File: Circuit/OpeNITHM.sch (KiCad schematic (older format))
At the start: 59 parts, among them J1 Conn_01x12, J2 Conn_01x12, J3 Conn_01x08, J4 Conn_01x11, J5 Conn_01x08, J6 Conn_01x11, J7 Conn_01x04

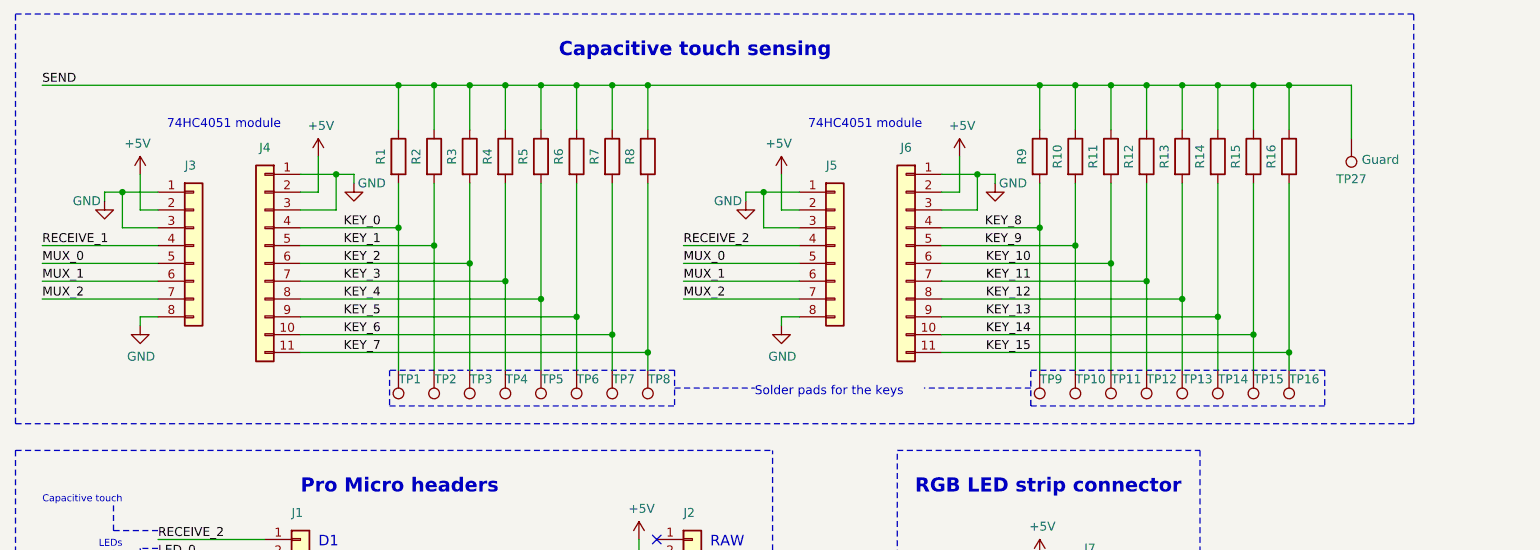
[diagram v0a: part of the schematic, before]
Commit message: Fix schematic files
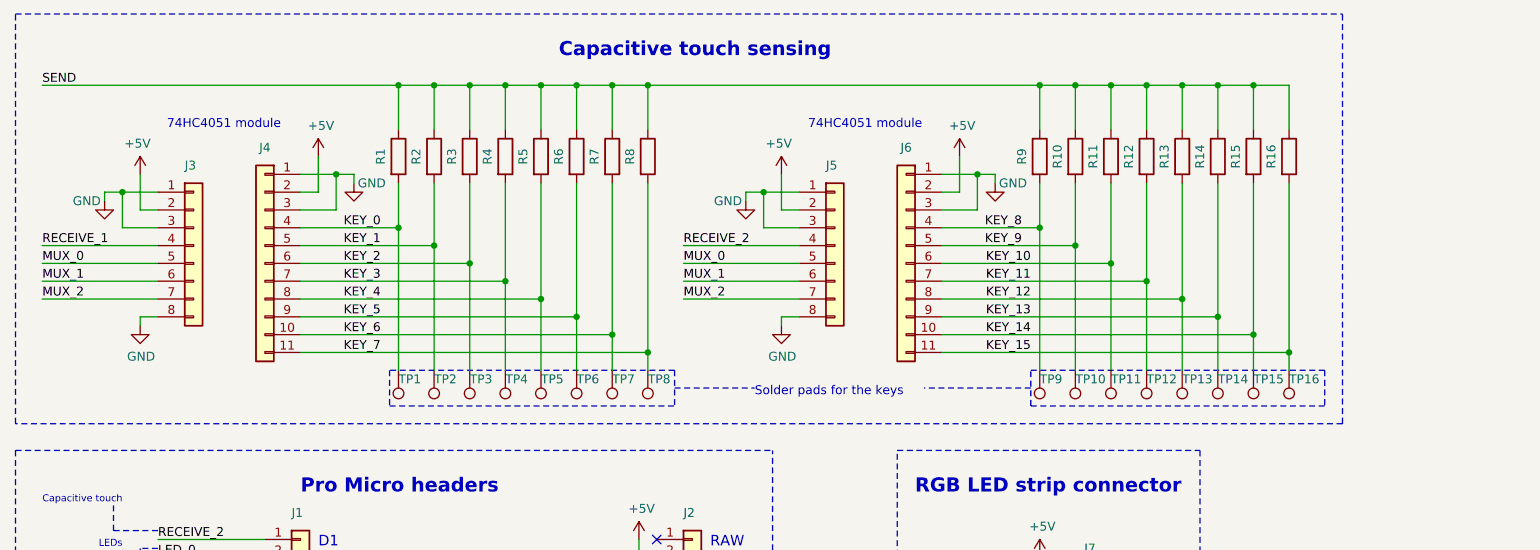
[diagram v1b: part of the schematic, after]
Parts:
- removed TP27: Guard, Connector_Wire:SolderWirePad_1x01_Drill1mm, symbol Connector:TestPoint
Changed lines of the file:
@@
 	9100 1200 9100 1450
+Wire Wire Line
+	9300 1200 9300 1450
 Wire Wire Line
 	9500 1200 9500 1450
@@
 Text Label 6100 2100 0    50   ~ 0
 RECEIVE_2
+Wire Wire Line
+	5900 1200 8100 1200
 Connection ~ 5900 1200
 Connection ~ 8100 1200
@@
 	3050 2550 3050 2500
 Wire Notes Line
-	10200 3100 10200 800
+	2350 800  9800 800
+Wire Notes Line
+	9800 3100 9800 800
+Wire Notes Line
+	9800 3100 2350 3100
 Wire Notes Line
 	2350 3100 2350 800
@@
 Wire Notes Line
 	2350 3250 6600 3250
-Wire Wire Line
-	5900 1200 8100 1200
-Wire Wire Line
-	9300 1200 9300 1450
-Connection ~ 9500 1200
-Wire Notes Line
-	2350 800  10200 800
-Wire Notes Line
-	2350 3100 10200 3100
-Wire Wire Line
-	9850 1200 9850 1500
-Wire Wire Line
-	9500 1200 9850 1200
-$Comp
-L Connector:TestPoint TP27
-U 1 1 5C685989
-P 9850 1500
-F 0 "TP27" H 9850 1756 50  0000 C TNN
-F 1 "Guard" H 9792 1618 50  0000 R CNN
-F 2 "Connector_Wire:SolderWirePad_1x01_Drill1mm" H 10050 1500 50  0001 C CNN
-F 3 "~" H 10050 1500 50  0001 C CNN
-	1    9850 1500
-	-1   0    0    1
-$EndComp
 $EndSCHEMATC
